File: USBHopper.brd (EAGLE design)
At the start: 85 x 20.3 mm, 42 parts, among them Q1 2.5A/30V, X1 USB-1X-2S-PLUG-A-SMD

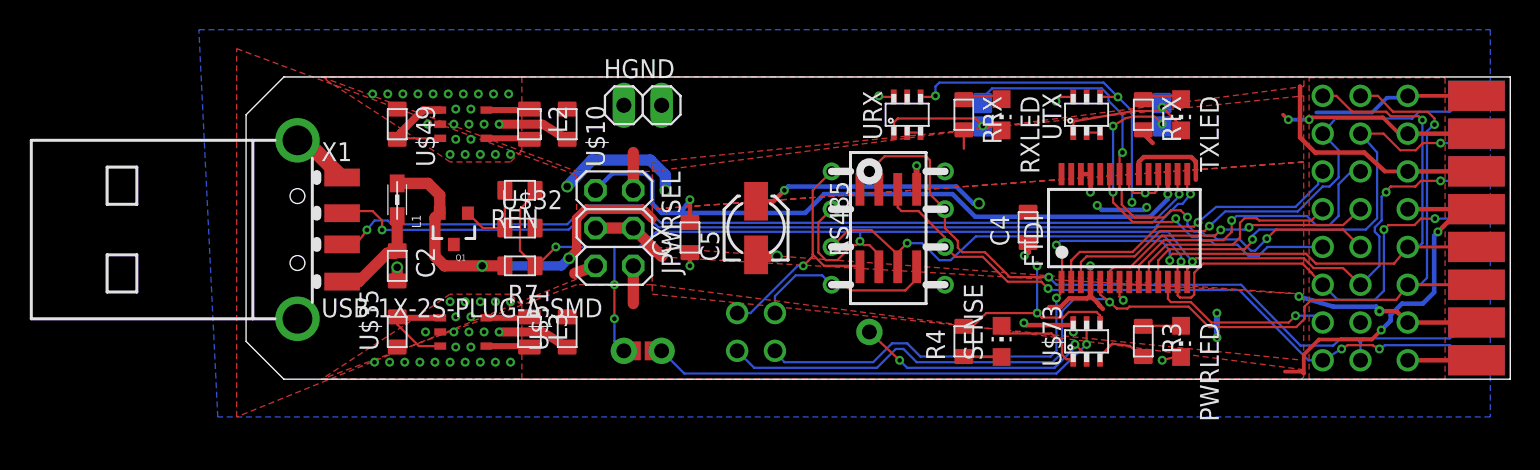
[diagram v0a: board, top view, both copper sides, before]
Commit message: Layout fertig. Logo!
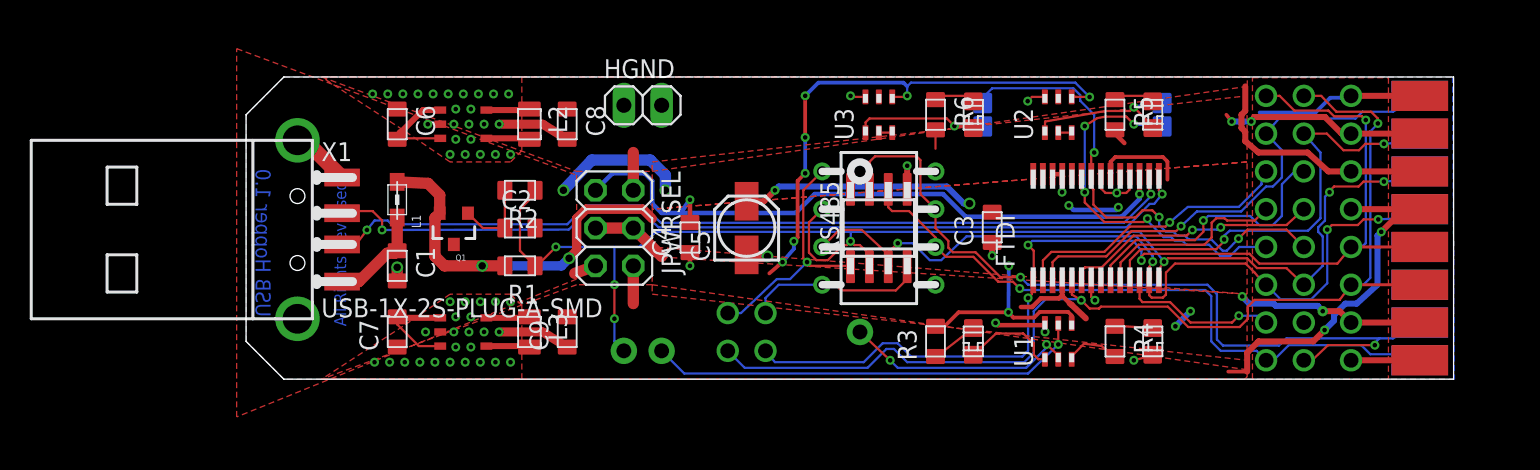
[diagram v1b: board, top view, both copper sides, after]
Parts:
- removed CX, U$32: 100nF, flo-parts:0805
- removed RRX, RTX: 270, flo-parts:0805
- removed U$73: (no value), flo-logic:SOT-457
- removed URX, UTX: 4k7/47k, flo-logic:SOT-457
- added C1: 10nF, flo-parts:0805
- added C3: 100nF, flo-parts:0805
- added R5, R6: 270, flo-parts:0805
- added U1: (no value), flo-logic:SOT-457
- added U2, U3: 4k7/47k, flo-logic:SOT-457
- C2: value 10nF -> 100nF
- FTDI: device ftdichip:SSOP28 -> ftdichip:SSOP28_FLO
- L1: device wuerth-elektronik:0805 -> wuerth_elektronik:0805
- PWRLED, RXLED, SENSE, TXLED: device led:CHIP-LED0805 -> flo-led:KPT-2012
- U$27: value CON1X2PIN_BRIDGE -> CON1X2PIN_XL; device flo-header:1X2PINS_BRIDGE -> flo-header:1X2PINS
- moved C4 22.7 mm to (29.8, 9.53)
- moved R3 14.0 mm to (46.4, 2.54), turned to 90 degrees
- moved R4 10.2 mm to (58.4, 2.54), turned to 270 degrees
- moved C2 8.64 mm to (18.4, 10.2), turned to 0 degrees
- moved U$64 3.81 mm to (74.3, 10.2)
- moved U$65 3.81 mm to (69.8, 10.2)
- moved U$66 3.81 mm to (80.8, 10.2)
- moved FTDI 1.91 mm to (57.1, 10.2)
- moved PWRLED 1.91 mm to (61.0, 2.54)
- moved TXLED 1.91 mm to (61.0, 17.8)
- moved RXLED 1.90 mm to (48.9, 17.8)
- moved SENSE 1.90 mm to (48.9, 2.54), turned to 180 degrees
- moved C5 0.63 mm to (33.7, 10.2)
- moved RS485 0.63 mm to (42.5, 10.2)
- moved U$19 0.63 mm to (33.7, 3.17)
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- renumbered R7 to R1, REN to R2, U$10 to C8, U$11 to U5, U$20 to U4, U$35 to C7, U$49 to C6, U$51 to C9
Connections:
- removed net N$5: URX.P$2, URX.P$3
- new net U3: U3.P$2, U3.P$3
- net +3V3OUT: now also C4.P$2; no longer CX.P$2
- net +5V: now also C2.P$2, R5.P$2, R6.P$2; no longer RRX.P$2, RTX.P$2, U$32.P$2
- net GND: now also C1.P$2, C3.P$1, PWRLED.2, U1.P$6, U2.P$6, U3.P$6; no longer C2.P$2, CX.P$1, PWRLED.C, U$73.P$6, URX.P$6, UTX.P$6
- net N$1: now also PWRLED.1, R4.P$1; no longer PWRLED.A, R3.P$1
- net N$10: now also TXLED.2, U2.P$1; no longer TXLED.C, UTX.P$1
- net N$11: now also R5.P$1, TXLED.1; no longer RTX.P$1, TXLED.A
- net N$12: now also R6.P$1, RXLED.1; no longer RRX.P$1, RXLED.A
- net N$13: now also R4.P$2, U1.P$3; no longer R3.P$2, U$73.P$3
- net N$14: now also U1.P$5; no longer U$73.P$5
- net N$2: now also R3.P$1, SENSE.1; no longer R4.P$1, SENSE.A
- net N$4: now also C1.P$1; no longer C2.P$1
- net N$6: now also RXLED.2, U3.P$1; no longer RXLED.C, URX.P$1
- net N$9: now also U2.P$2, U2.P$3; no longer UTX.P$2, UTX.P$3
- net PWREN: now also C2.P$1; no longer U$32.P$1
- net RX: now also U3.P$5; no longer URX.P$5
- net SENSE: now also U1.P$2; no longer U$73.P$2
- net SENSLED: now also SENSE.2, U1.P$1; no longer SENSE.C, U$73.P$1
- net TX: now also U2.P$5; no longer UTX.P$5
- net USB+5V: now also C3.P$2, R3.P$2, U1.P$4; no longer C4.P$2, R4.P$2, U$73.P$4
- net VCCIO: now also U2.P$4, U3.P$4; no longer URX.P$4, UTX.P$4
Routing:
- net VCCIO: track 49.6 -> 62.4 mm, vias 8 -> 11
- net PWREN#: track 96.4 -> 92.6 mm
- net RXLED#: track 36.3 -> 32.5 mm
- net RXD: track 76.9 -> 73.5 mm
- net TXDEN: track 58.7 -> 55.4 mm
- net TXD: track 75.0 -> 71.8 mm
- net RS485B: track 52.3 -> 54.7 mm, vias 1 -> 2
- net CTS#: track 32.2 -> 30.3 mm
- net RI#: track 19.3 -> 17.4 mm
- net DTR#: track 21.1 -> 19.2 mm
- net DCD#: track 15.2 -> 13.3 mm
- net CBUS4: track 12.6 -> 10.7 mm
- net USBDP: track 61.3 -> 59.4 mm
- net RTS#: track 35.7 -> 33.8 mm
- net N$14: track 31.4 -> 29.5 mm
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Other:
- board size 85 x 20.3 mm -> 81.2 x 20.3 mm
- board text added: "+ B A -"
- board text added: "1"
- board text added: "14"
- board text added: "15"
- board text added: "1v8"
- board text added: "2"
- board text added: "28"
- board text added: "3"
- board text added: "3v3"
- board text added: "4"
- board text added: "42"
- board text added: "485"
- board text added: "5"
- board text added: "8"
- board text added: "=HOT="
- board text added: "?"
- board text added: "All Rights Reversed"
- board text added: "BETA"
- board text added: "C1"
- board text added: "C2"
- board text added: "C3"
- board text added: "C4"
- board text added: "C5"
- board text added: "C6"
- board text added: "C7"
- board text added: "C8"
- board text added: "C9"
- board text added: "DI"
- board text added: "DM"
- board text added: "DP"
- board text added: "ENTER YOUR NAME HERE"
- board text added: "GND"
- board text added: "HOT END"
- board text added: "L1"
- board text added: "L2"
- board text added: "L3"
- board text added: "MOTHER BOARD"
- board text added: "NOW YOU SEE ME"
- board text added: "PUNK"
- board text added: "R1"
- board text added: "R2"
- board text added: "R3"
- board text added: "R4"
- board text added: "R5"
- board text added: "R6"
- board text added: "RO"
- board text added: "RO RE DE DI"
- board text added: "RXD CTS DSR RI CB1 CB3 GND B"
- board text added: "S"
- board text added: "TXD RTS DTR DCD CB0 CB2 CB4 A"
- board text added: "U1"
- board text added: "U2"
- board text added: "U3"
- board text added: "U4"
- board text added: "U5"
- board text added: "VCC"
- board text added: "binary"
- board text added: "is not"
- board text added: "kitchen"
- board text added: "www.binary-kitchen.de"
- board text removed: "+1v8"
- board text removed: "+3v3"
- board text removed: "+5v"
- board text removed: "- +"
- board text removed: "INT"
- board text removed: "usb+5v"
- board text removed: "vccio"
